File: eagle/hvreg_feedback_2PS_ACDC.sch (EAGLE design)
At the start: 18 parts

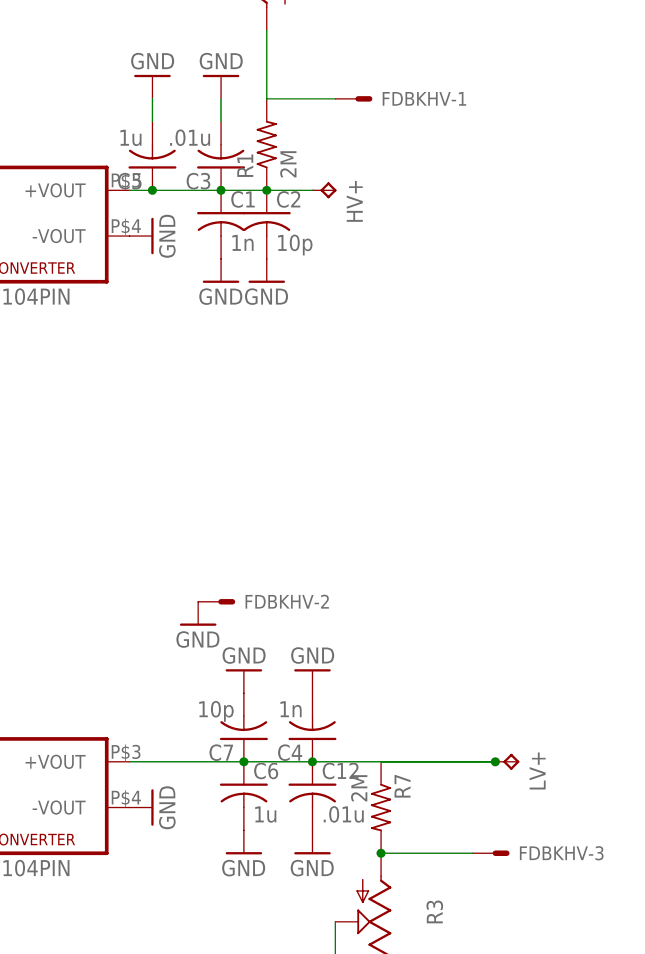
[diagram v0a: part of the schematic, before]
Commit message: IXYS board solution, gatedriver components
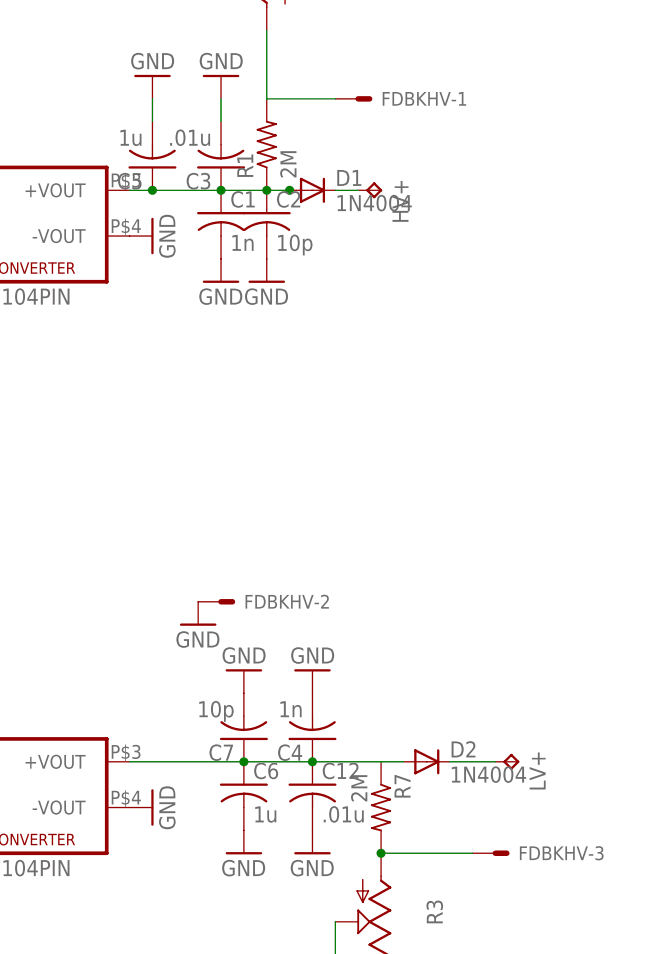
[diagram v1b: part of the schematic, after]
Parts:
- added D1, D2: 1N4004, diode:1N4004
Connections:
- new net N$6: D1.C, HV+.TP
- new net N$7: D2.C, LV+.TP
- net N$1: now also D1.A; no longer HV+.TP
- net N$2: now also D2.A; no longer LV+.TP
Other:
- moved on the sheet: HV+
